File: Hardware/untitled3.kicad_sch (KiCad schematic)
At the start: 0 parts

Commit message: CHECK
CHECK1
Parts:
- added A3144: ~, symbol thinh:A3144_
- added C15, C19, C21: 0.1uF, symbol Triet_KiCAD_Sym:CAP_POL
- added C16, C18, C22: 0.22uF, symbol Triet_KiCAD_Sym:CAP_POL
- added C17: 100nF, symbol Triet_KiCAD_Sym:CAP_CER
- added C20: 2.2uF, symbol Triet_KiCAD_Sym:CAP_POL
- added C23: 10uF, symbol Triet_KiCAD_Sym:CAP_POL
- added C24: 47uF, symbol Triet_KiCAD_Sym:CAP_POL
- added GP2Y1010AU0F1: ~, symbol GP2Y1010AU0F:GP2Y1010AU0F
- added HPP845E034R1: ~, symbol HPP845E034R5:HPP845E034R5_
- added R1, R10, R8: 10k, symbol Triet_KiCAD_Sym:Res
- added R11, R9: 4.7k, symbol Triet_KiCAD_Sym:Res
- added R13, R14, R15, R16: 100R, symbol Triet_KiCAD_Sym:Res
- added R3, R7: N.M, symbol Triet_KiCAD_Sym:Res
- added U2: BM1383AGLV-ZE2, symbol BM1383AGLV:BM1383AGLV-ZE2
- added U4: HMC5883L, HMC5883L:LPCC-16, symbol HMC5883L_1:HMC5883L
- added U6: AS5600, symbol AS5600:AS5600
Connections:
- new net: R14.1, U6.7 (SCL)
- new net: C18.2, U2.1 (DREG)
- new net: C22.1, U4.8 (SETP)
- new net: C22.2, U4.12 (SETC)
- new net: HPP845E034R1.1 (DATA), R10.2
- new net: HPP845E034R1.6 (SCK), R8.2
- new net: C24.1, GP2Y1010AU0F1.1 (V-LED), R16.2
- new net: R9.1, U4.1 (SCL)
- new net: C16.1, U4.10 (C1)
- new net: C19.2, U4.13 (VDDIO)
- new net: R11.1, U4.16 (SDA)
- new net: C20.2, U4.2 (VDD)
- new net: C21.2, U4.4 (S1)
- new net: R15.1, U6.6 (SDA)
- new net: R13.2, U6.8 (DIR)
- new net: U2.4 (TIN), U2.5 (TOUT)
- new net 3V3: C15.2, C17.1, C19.1, C20.1, C21.1, C23.1, HPP845E034R1.5 (VDD), R10.1, R13.1, R14.2, R15.2, R3.1, R3.2, R7.1, R7.2, R8.1, U2.10 (SDA), U2.2 (VDD), U2.9 (SCL), U6.2 (VDD3V3)
- new net 5V: A3144.1 (Vcc), GP2Y1010AU0F1.6 (Vcc), R1.1, R16.1
- new net C1IND: GP2Y1010AU0F1.5 (Vo)
- new net DRDY: U2.11 (DRDY), U4.15 (DRDY)
- new net GND: A3144.2 (GND), C15.1, C16.2, C17.2, C18.1, C23.2, C24.2, GP2Y1010AU0F1.2 (LED-GND), GP2Y1010AU0F1.4 (S-GND), HPP845E034R1.2 (GND), U2.12 (TEST0), U2.3 (VSS), U2.6 (TEST1), U4.11 (GND@2), U4.9 (GND@1), U6.4 (GND)
- new net RA0: GP2Y1010AU0F1.3 (LED)
- new net RA1: A3144.3 (Signal), R1.2
- new net SCL2: R9.2
- new net SDA2: R11.2
- no-connect marks 0 -> 3
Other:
- note added: "Dust Sensor"
- note added: "Hall Sensor"
- note added: "Pressure Sensor"
- note added: "Rainfall Sensor"
- note added: "Temperature & Humidity Sensor"
- note added: "Wind Direction Sensor"

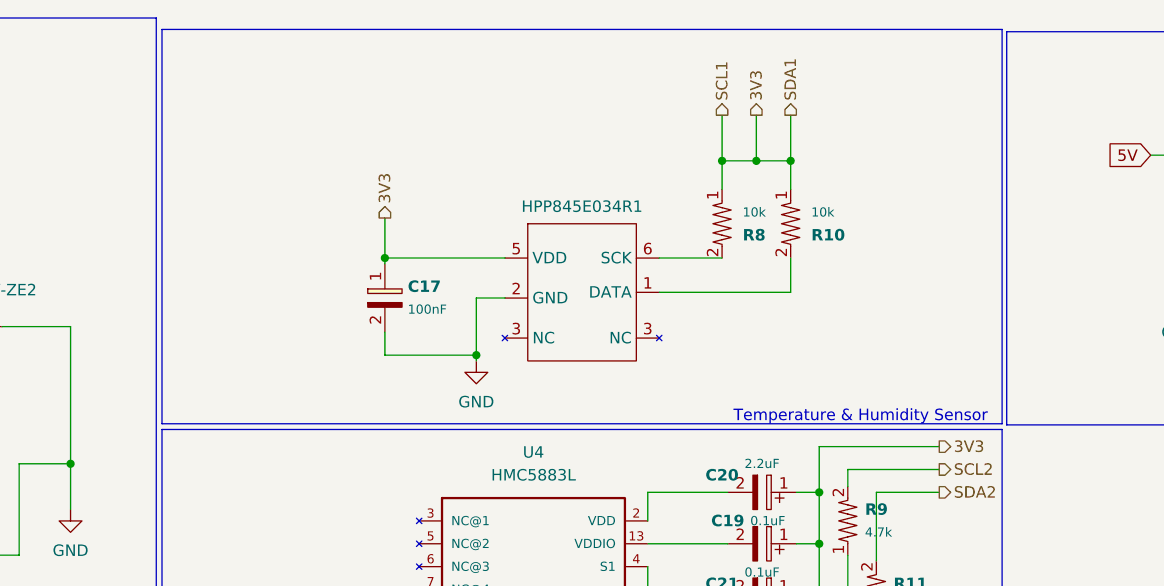
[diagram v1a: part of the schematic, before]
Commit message: CHECK
CHECK
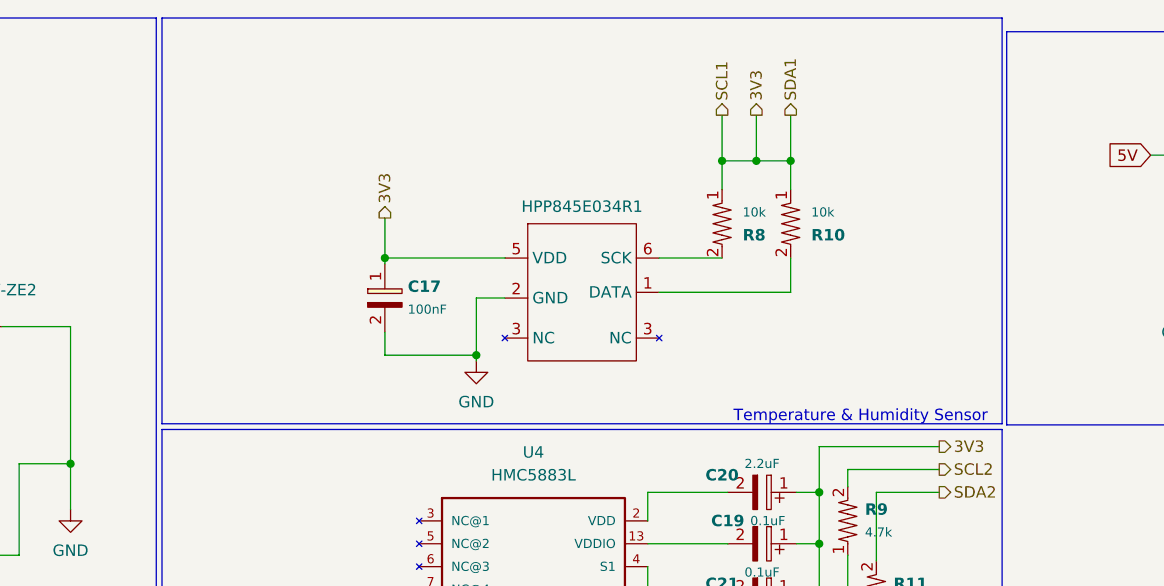
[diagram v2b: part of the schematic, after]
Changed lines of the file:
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@@
     (fill (type none))
   )
-  (rectangle (start 122.555 13.97) (end 215.9 57.785)
+  (rectangle (start 122.555 12.7) (end 215.9 57.785)
     (stroke (width 0) (type default))
     (fill (type none))
